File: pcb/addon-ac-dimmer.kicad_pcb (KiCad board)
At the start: 2 copper layers, 45.5 x 45.3 mm, 40 parts, among them J1 Screw_Terminal_01x05, J2 Conn_01x02_Male ZMCT, J3 Conn_01x05_Male, J4 Conn_01x05_Male RIGHT, J5 Programm header, Q1 BT136-600D, Q2 BT136-600D, Q5 2N3904, U1 HLK-PM02, U2 MOC3052, U3 MOC3052, U4 4N35, U6 ATTINY414-SSNR, U7 H11AA1SM

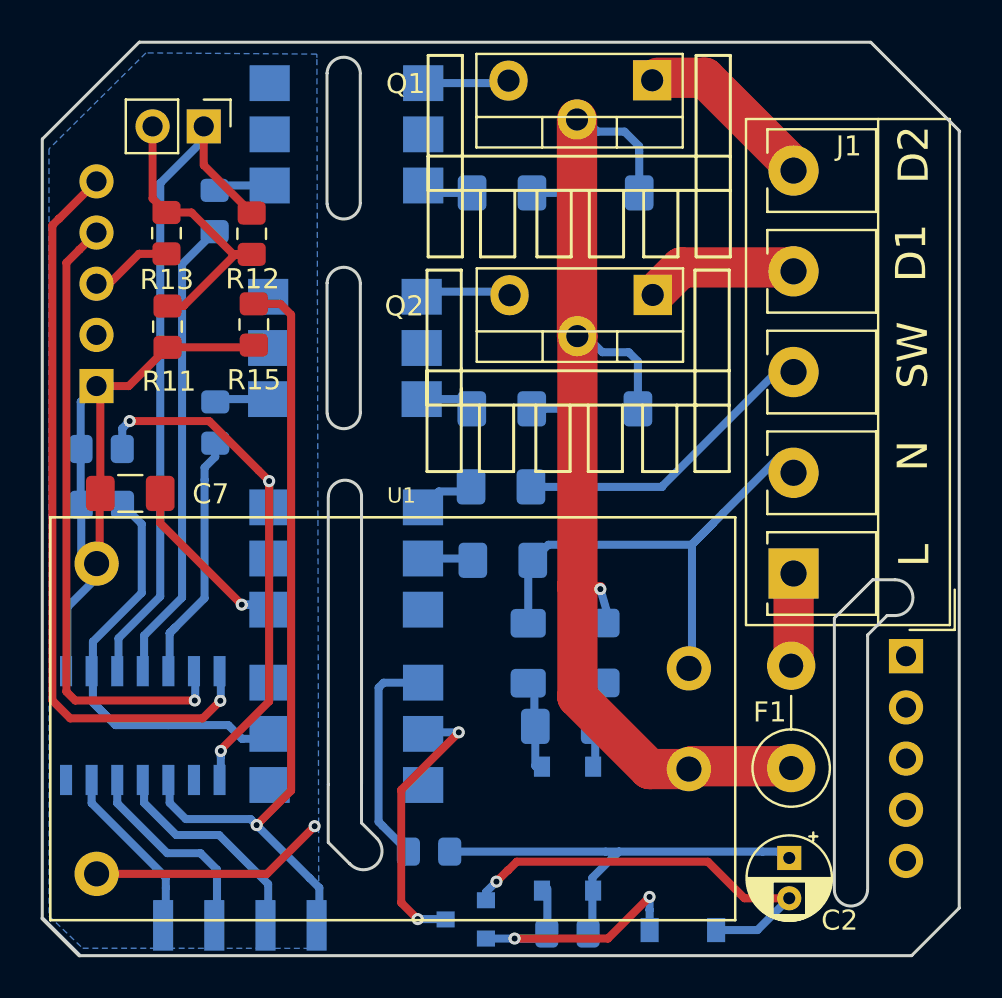
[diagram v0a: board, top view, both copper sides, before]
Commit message: Repository cleanup
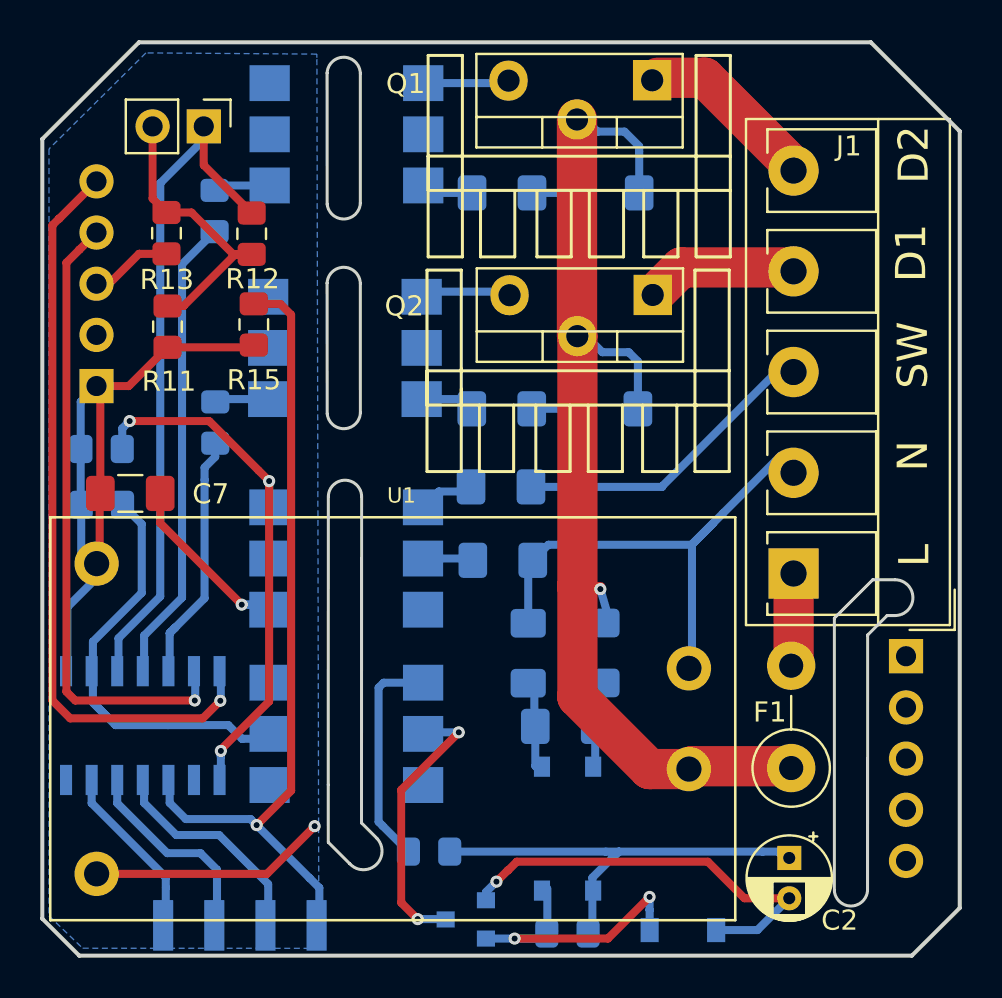
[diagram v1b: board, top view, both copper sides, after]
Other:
- outline, holes or cut-outs redrawn
